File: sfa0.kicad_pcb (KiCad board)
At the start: 2 copper layers, 30.8 x 26 mm, 30 parts, among them J1 AudioJack4, J2 AudioJack4, U1 AP2112K-3.3, U2 AP2112K-1.2, U3 ICE40UP5K-SG48ITR, U4 W25Q128JVS, X1 ASDMB-xxxMHz

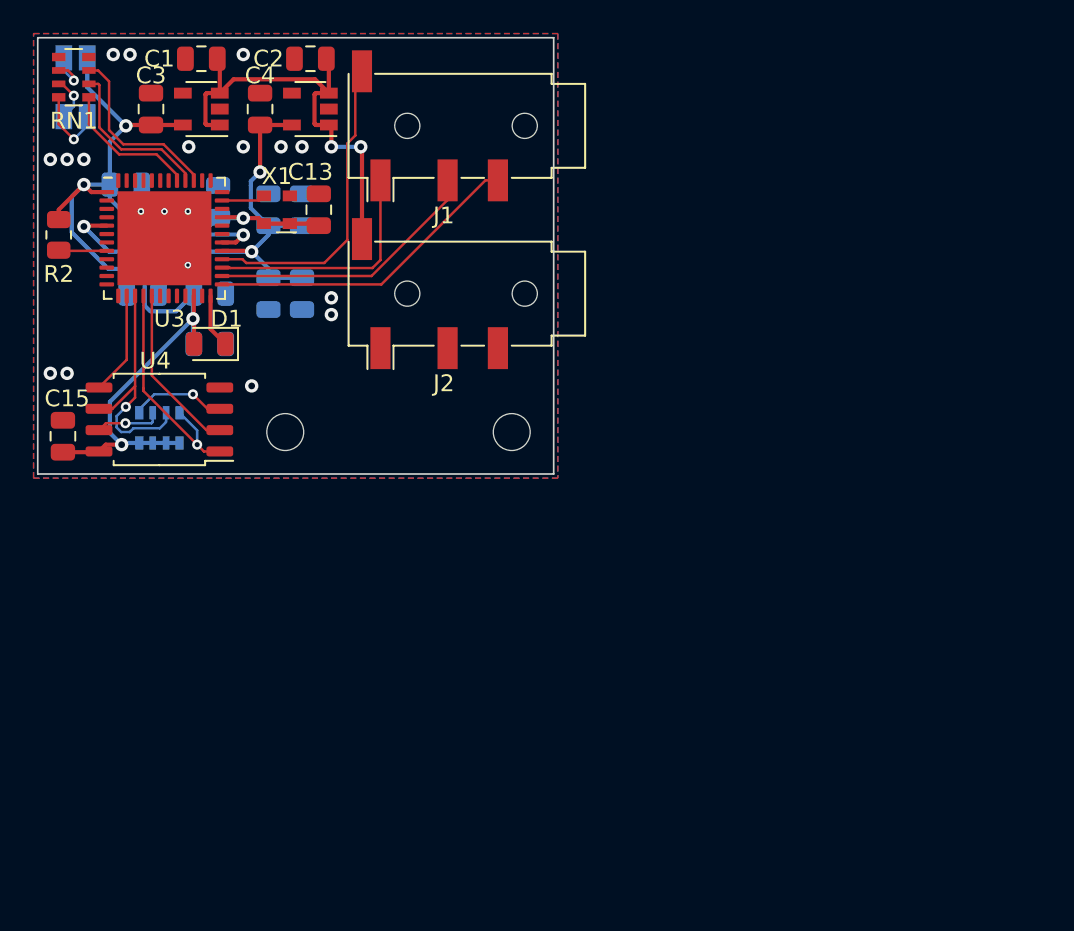
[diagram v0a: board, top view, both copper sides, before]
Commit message: redesign
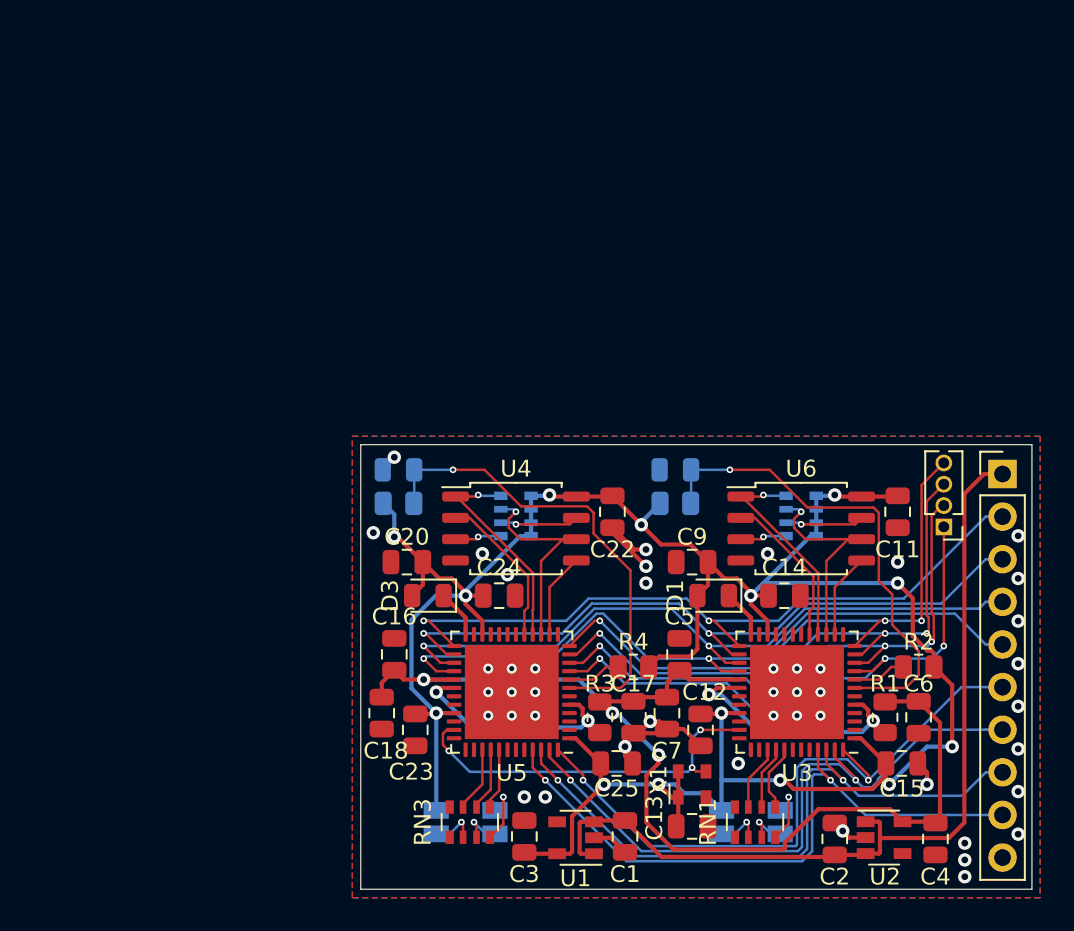
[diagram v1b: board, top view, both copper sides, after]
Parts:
- removed C10: 100u, Capacitor_SMD:C_0805_2012Metric
- removed C8: 10u, Capacitor_SMD:C_0805_2012Metric
- removed H1, H2: MountingHole, MountingHole:MountingHole_2.2mm_M2
- added C16: 100u, Capacitor_SMD:C_0805_2012Metric, F.Cu at (132.5, 99.0)
- added C17: 100u, Capacitor_SMD:C_0805_2012Metric, F.Cu at (146.8, 102.8)
- added C18: 10u, Capacitor_SMD:C_0805_2012Metric, F.Cu at (131.8, 102.5)
- added C20: 100u, Capacitor_SMD:C_0805_2012Metric, F.Cu at (133.2, 93.5)
- added C22: 100u, Capacitor_SMD:C_0805_2012Metric, F.Cu at (145.5, 90.5)
- added C23: 100u, Capacitor_SMD:C_0805_2012Metric, F.Cu at (133.8, 103.5)
- added C24: 100u, Capacitor_SMD:C_0805_2012Metric, F.Cu at (138.8, 95.5)
- added C25: 100u, Capacitor_SMD:C_0805_2012Metric, F.Cu at (145.8, 105.5)
- added D3: D_Schottky, Diode_SMD:D_0805_2012Metric, F.Cu at (134.5, 95.5)
- added D4: LED_RGBA, LED_SMD:LED_RGB_1210, B.Cu at (136.8, 109.0)
- added D5: BLU, LED_SMD:LED_0805_2012Metric, B.Cu at (132.8, 88.0)
- added D6: BLU, LED_SMD:LED_0805_2012Metric, B.Cu at (149.2, 88.0)
- added R3: 100R, Resistor_SMD:R_0805_2012Metric, F.Cu at (144.8, 102.8)
- added R4: 10K, Resistor_SMD:R_0805_2012Metric, F.Cu at (146.8, 99.8)
- added R5: 2K2, Resistor_SMD:R_0805_2012Metric, B.Cu at (132.8, 90.0)
- added R6: 2K2, Resistor_SMD:R_0805_2012Metric, B.Cu at (149.2, 90.0)
- added RN3: 330R, Resistor_SMD:R_Array_Convex_4x0603, F.Cu at (137.0, 109.0)
- added RN4: 10K, Resistor_SMD:R_Array_Convex_4x0603, B.Cu at (139.8, 90.8)
- added U5: ICE40UP5K-SG48ITR, Package_DFN_QFN:QFN-48-1EP_7x7mm_P0.5mm_EP5.6x5.6mm, F.Cu at (139.5, 101.2)
- added U6: W25Q32JVSS, Package_SO:SOIC-8_5.23x5.23mm_P1.27mm, F.Cu at (156.8, 91.5)
- C11: value 10u -> 100u; moved to F.Cu
- C12, C14, C5, C6, C9, R1: moved to F.Cu
- C7: value 100u -> 10u; moved to F.Cu
- J1: value AudioJack4 -> Conn_01x10_Male; footprint Connector_Audio:Jack_3.5mm_PJ320D_Horizontal -> Connector_PinHeader_2.54mm:PinHeader_1x10_P2.54mm_Vertical
- J2: value AudioJack4 -> Conn_01x04_Male; footprint Connector_Audio:Jack_3.5mm_PJ320D_Horizontal -> Connector_PinHeader_1.27mm:PinHeader_1x04_P1.27mm_Vertical
- U4: value W25Q128JVS -> W25Q32JVSS
- moved RN1 60.2 mm to (154.0, 109.0), turned to 90 degrees
- moved D2 59.5 mm to (153.8, 109.0), turned to 180 degrees
- moved C4 59.3 mm to (164.8, 110.0), turned to 270 degrees
- moved R2 57.4 mm to (163.8, 99.8), turned to 180 degrees
- moved C2 56.0 mm to (158.8, 110.0), turned to 90 degrees
- moved U2 55.3 mm to (161.7, 109.9), turned to 0 degrees
- moved C15 53.7 mm to (162.8, 105.5), turned to 0 degrees
- moved C1 52.8 mm to (146.2, 109.8), turned to 270 degrees
- moved R1 52.2 mm to (161.8, 102.8), turned to 90 degrees
- moved C6 49.2 mm to (163.8, 102.8), turned to 270 degrees
- moved U1 48.8 mm to (143.3, 109.9)
- moved C3 48.7 mm to (140.2, 109.8)
- moved U3 46.4 mm to (156.5, 101.2), turned to 180 degrees
- moved C14 46.3 mm to (155.8, 95.5)
- moved C13 43.0 mm to (150.2, 109.2), turned to 0 degrees
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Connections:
- net /RGB_B renamed /Core2/RGB_B
- net /RGB_G renamed /Core2/RGB_G
- net /RGB_R renamed /Core2/RGB_R
- net Net-(R2-Pad2) renamed /Core2/RESET
- C11 pad 1: +1V2 -> +3V3
- C5 pad 1: +3V3 -> +1V2
- C9 pad 1: +1V2 -> +3V3
- RN2 pad 7: /FLASH_SCK -> /Core2/FLASH_SCK
- RN2 pad 8: /FLASH_SS -> /Core2/FLASH_SS
- U3 pad 10: Net-(U3-Pad10) -> /C2
- U3 pad 11: Net-(U3-Pad11) -> /C3
- U3 pad 12: Net-(U3-Pad12) -> /C4
- U3 pad 14: /FLASH_MOSI -> /Core2/FLASH_MOSI
- U3 pad 15: /FLASH_SCK -> /Core2/FLASH_SCK
- U3 pad 16: /FLASH_SS -> /Core2/FLASH_SS
- U3 pad 17: /FLASH_MISO -> /Core2/FLASH_MISO
- U3 pad 25: /CONN_D2 -> /D1
- U3 pad 26: /CONN_D3 -> /D2
- U3 pad 27: /CONN_D4 -> /D3
- U3 pad 28: /CONN_D1 -> /D4
- U3 pad 45: Net-(U3-Pad45) -> /D8
- U3 pad 46: Net-(U3-Pad46) -> /D7
- U3 pad 47: Net-(U3-Pad47) -> /D6
- U3 pad 48: Net-(U3-Pad48) -> /D5
- U3 pad 7: Net-(U3-Pad7) -> /Core2/DONE
- U3 pad 9: Net-(U3-Pad9) -> /C1
- U4 pad 1: /FLASH_SS -> /Core1/FLASH_SS
- U4 pad 2: /FLASH_MISO -> /Core1/FLASH_MISO
- U4 pad 3: Net-(RN2-Pad5) -> Net-(RN4-Pad5)
- U4 pad 5: /FLASH_MOSI -> /Core1/FLASH_MOSI
- U4 pad 6: /FLASH_SCK -> /Core1/FLASH_SCK
- U4 pad 7: Net-(RN2-Pad6) -> Net-(RN4-Pad6)
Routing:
- net +3V3: track 70.5 -> 158.4 mm, vias 5 -> 14
- net /D1: track 0.00 -> 43.0 mm, vias 0 -> 2
- net /D4: track 0.00 -> 42.8 mm, vias 0 -> 2
- net /D2: track 0.00 -> 42.5 mm, vias 0 -> 2
- net /D3: track 0.00 -> 41.9 mm, vias 0 -> 2
- net +1V2: track 26.4 -> 66.1 mm, vias 2 -> 3
- net /D8: track 0.00 -> 39.2 mm, vias 0 -> 2
- net /D5: track 0.00 -> 39.2 mm, vias 0 -> 2
- net /D6: track 0.00 -> 39.0 mm, vias 0 -> 2
- net /D7: track 0.00 -> 38.8 mm, vias 0 -> 2
- net /C4: track 0.00 -> 36.3 mm, vias 0 -> 3
- net /C2: track 0.00 -> 36.1 mm, vias 0 -> 3
- net /C3: track 0.00 -> 35.9 mm, vias 0 -> 3
- net /C1: track 0.00 -> 35.8 mm, vias 0 -> 3
- net /Core2/DONE: track 0.00 -> 29.0 mm, vias 0 -> 1
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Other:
- board size 30.8 x 26 mm -> 40 x 26.5 mm
- net class Default: via_dia 0.6 -> 0.4; via_drill 0.3 -> 0.2
